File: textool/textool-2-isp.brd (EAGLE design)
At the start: 54.3 x 42.5 mm, 4 parts

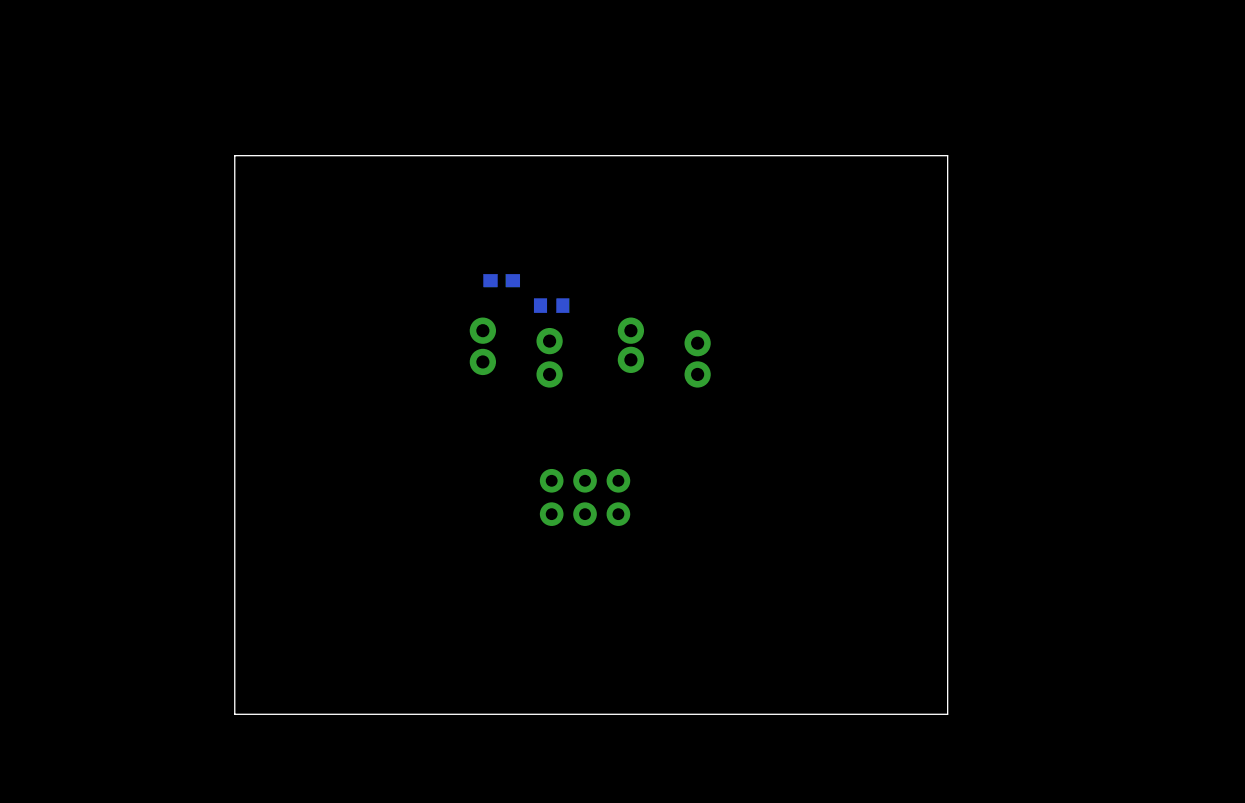
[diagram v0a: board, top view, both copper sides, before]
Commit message: fixes, design improvements
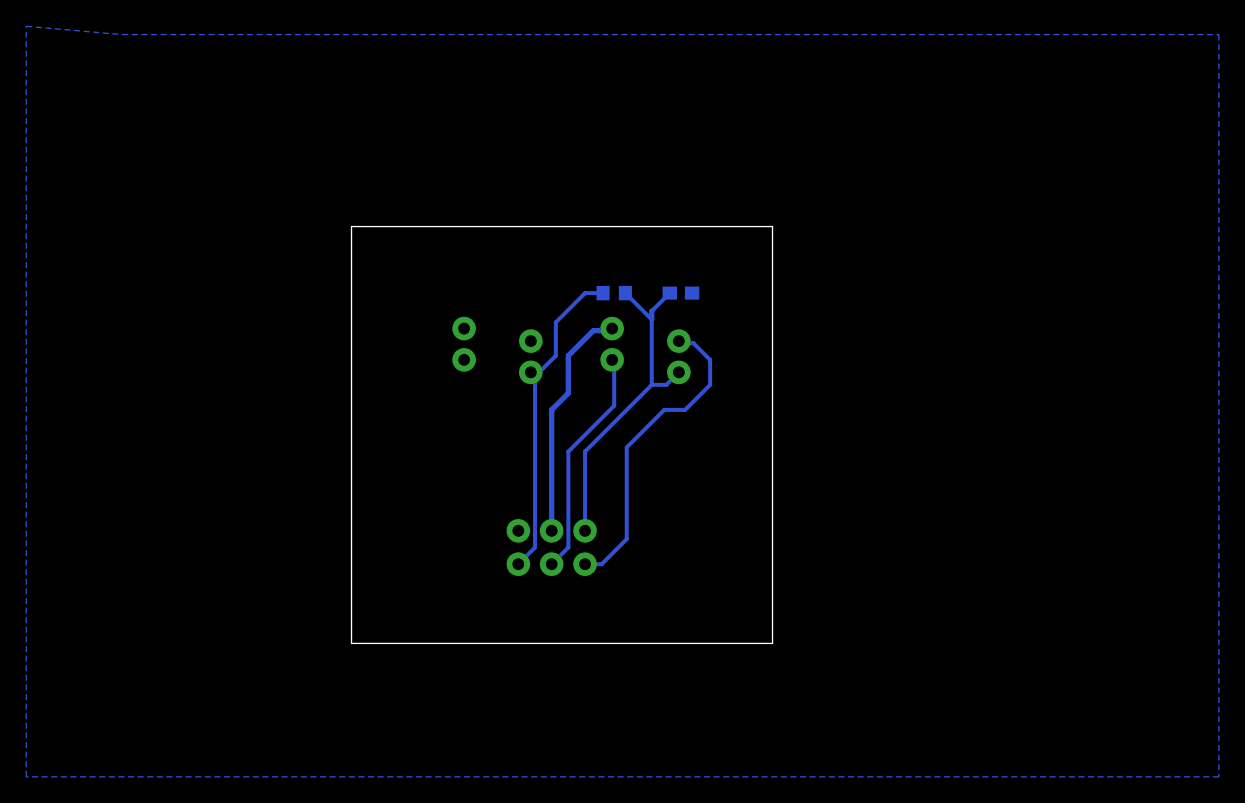
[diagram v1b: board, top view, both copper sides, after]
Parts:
- moved C1 13.7 mm to (30.8, 25.7)
- moved R1 4.86 mm to (25.7, 25.7), turned to 0 degrees
- moved ISP1 4.58 mm to (21.0, 6.35), turned to 90 degrees
- moved U$1 0.90 mm to (22.9, 21.0), turned to 180 degrees
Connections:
- net GND: now also U$1.P$5; no longer U$1.P$4
- net MISO: now also U$1.P$3; no longer U$1.P$6
- net MOSI: now also U$1.P$4; no longer U$1.P$5
- net RST: now also U$1.P$8; no longer U$1.P$1
- net SCK: now also U$1.P$2; no longer U$1.P$7
- net VCC: now also U$1.P$1; no longer U$1.P$8
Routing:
- net VCC: track 0.00 -> 26.1 mm
- net RST: track 0.00 -> 24.7 mm
- net MISO: track 0.00 -> 24.1 mm
- net MOSI: track 0.00 -> 18.0 mm
- net SCK: track 0.00 -> 17.6 mm
- added copper zone on layer 16, net GND
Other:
- board size 54.3 x 42.5 mm -> 32.1 x 31.7 mm
